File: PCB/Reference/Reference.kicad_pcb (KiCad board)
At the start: 2 copper layers, 70 x 70 mm, 31 parts, among them J1 Conn_01x04, U1 LMR16006XDDCR, U2 MD8942, U3 Barcode

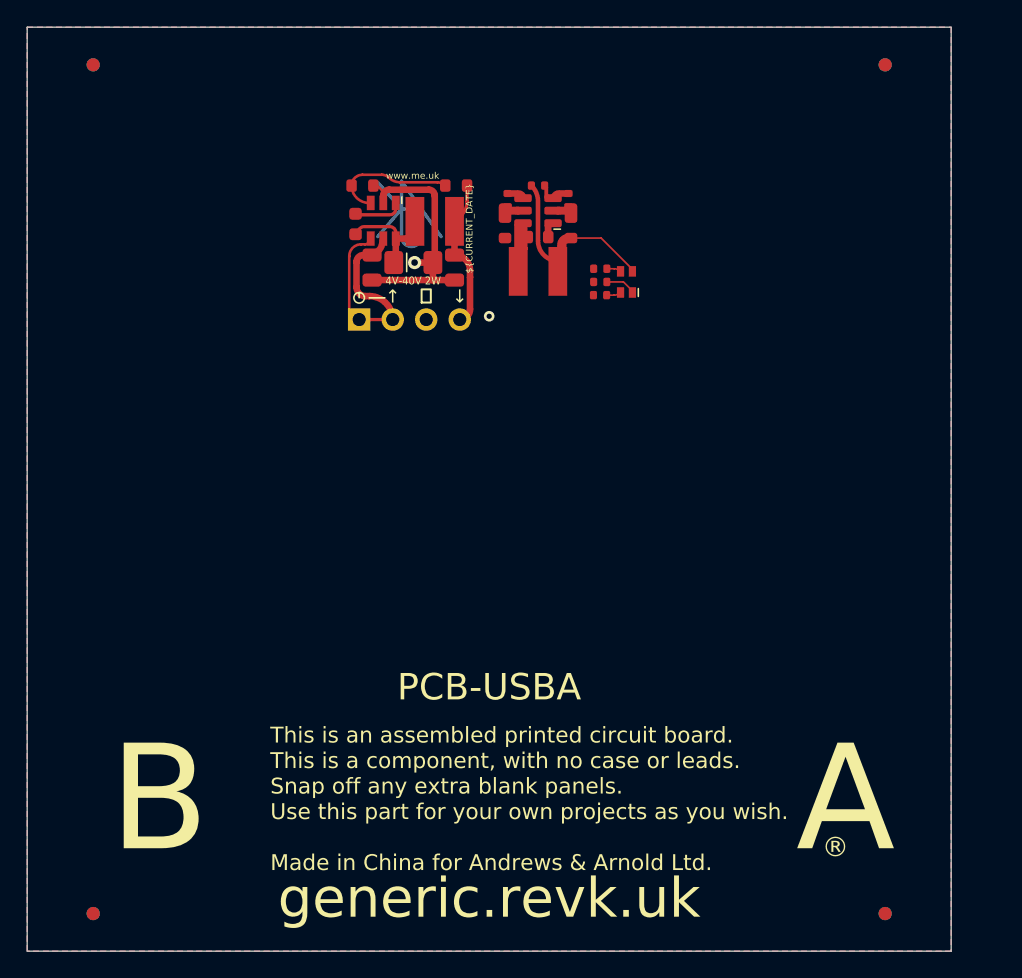
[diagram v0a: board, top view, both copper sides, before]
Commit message: PCB templatge
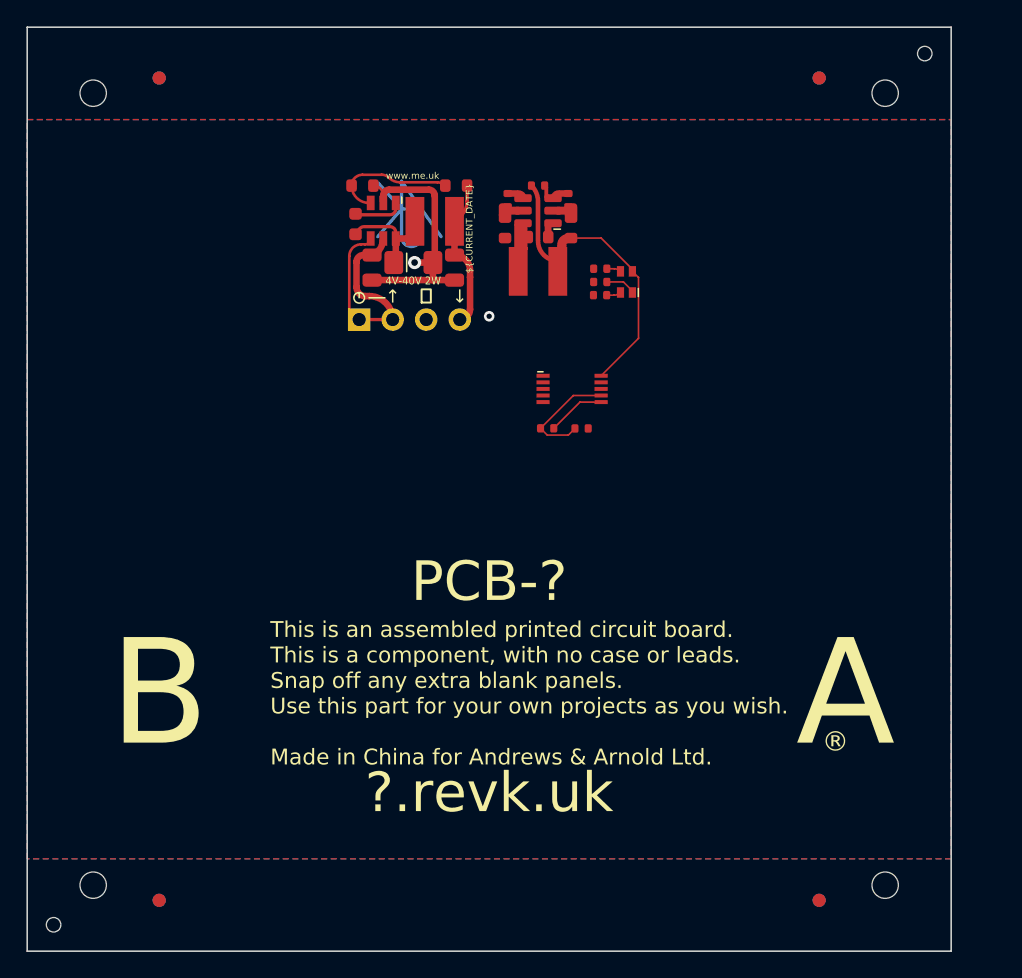
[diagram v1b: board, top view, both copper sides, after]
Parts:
- removed FID1, FID2, FID3, FID4, FID5, FID6, FID7, FID8: Fiducial, Fiducial:Fiducial_1mm_Mask2mm
- added C7: 0.1uF, RevK:C_0402, F.Cu at (142.0, 60.4)
- added PCB1: 70x70, RevK:PCB7070, F.Cu at (135.0, 65.0)
- added R9: 4k7, RevK:R_0402, F.Cu at (139.4, 60.4)
- added U4: CH340X, RevK:CH340X, F.Cu at (141.3, 57.4)
- moved U3 9.45 mm to (153.5, 64.0)
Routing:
- net +3.3V: track 5.77 -> 23.7 mm
- net BOOT: track 0.00 -> 4.41 mm
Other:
- board text added: "?.revk.uk"
- board text added: "PCB-?"
- board text removed: "PCB-USBA"
- board text removed: "generic.revk.uk"
